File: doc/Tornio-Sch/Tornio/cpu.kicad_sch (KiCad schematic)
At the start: 24 parts, among them J3 Program, J5 Conn_02x20_Odd_Even, J7 Conn_02x07_Odd_Even, U10 STM32F103C6Tx, U2 ULN2003, U9 AMS1117-3.3, Y2 12MHz

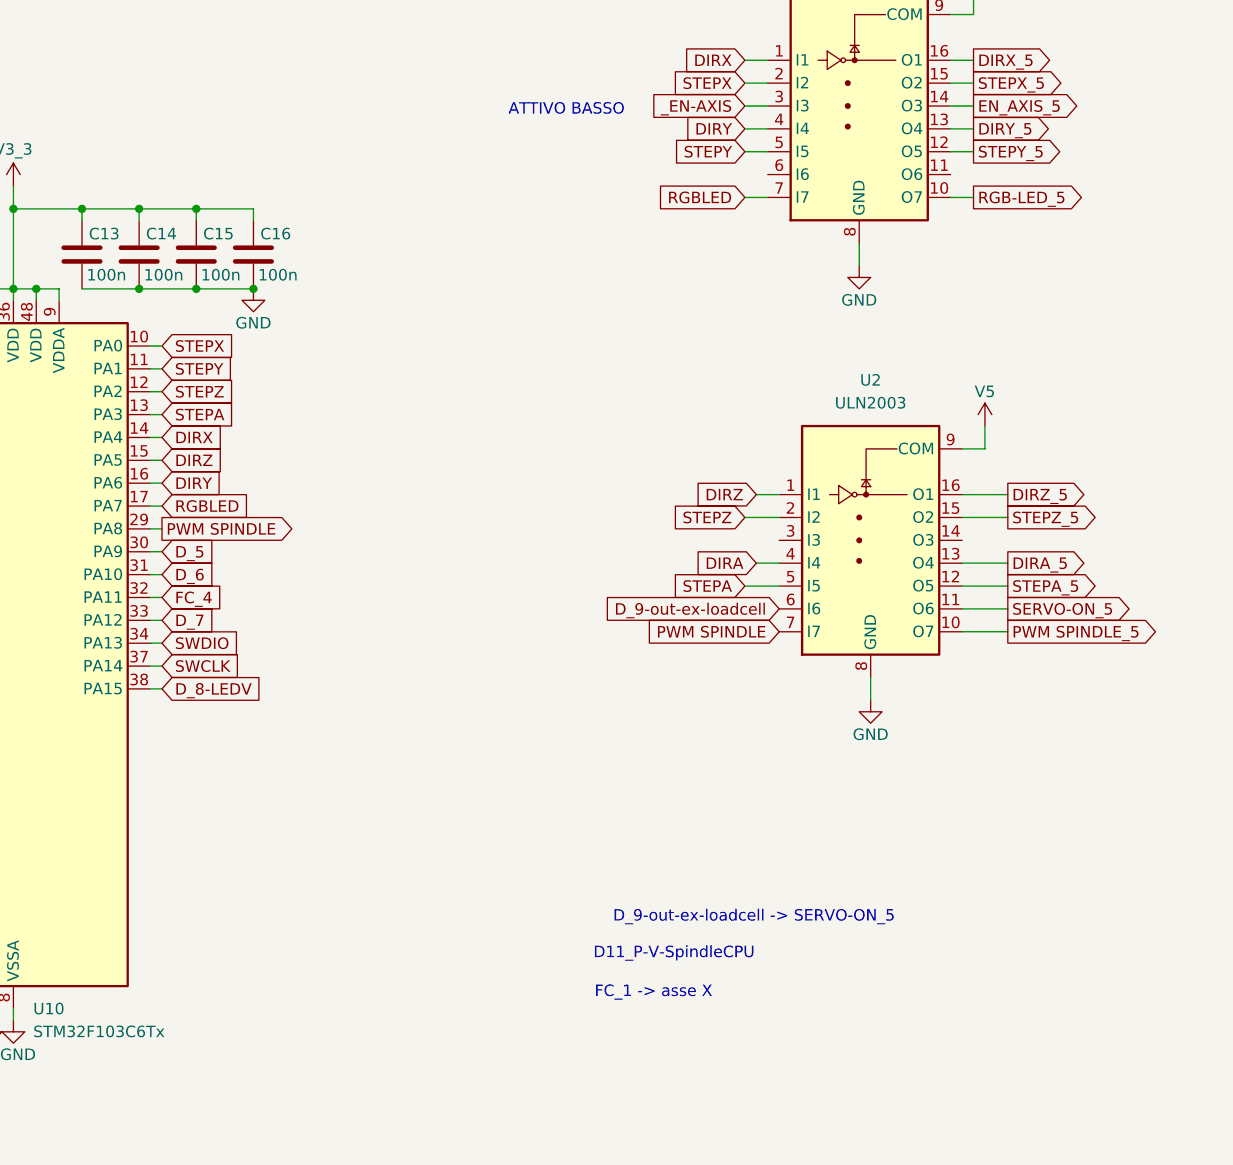
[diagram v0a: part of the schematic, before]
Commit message: eliminati file tenda da sole da accessori
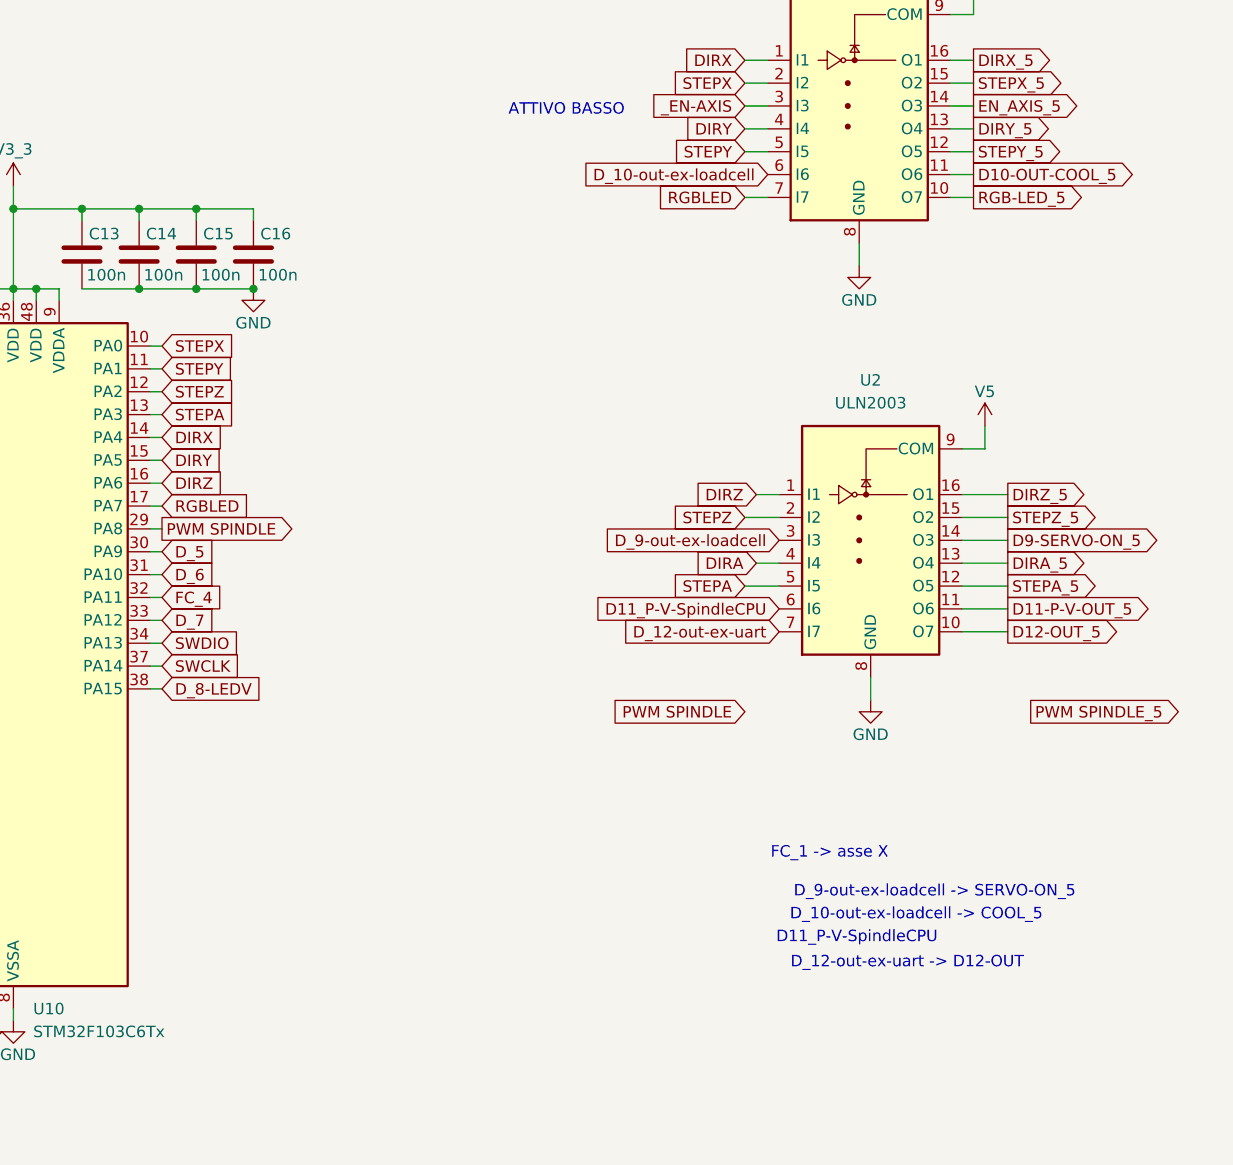
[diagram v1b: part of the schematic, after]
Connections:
- net D11_P-V-SpindleCPU: now also U2.6 (I6)
- net DIRY: now also U10.15 (PA5); no longer U10.16 (PA6)
- net DIRZ: now also U10.16 (PA6); no longer U10.15 (PA5)
- net D_10-out-ex-loadcell: now also U2.6 (I6)
- net D_12-out-ex-uart: now also U2.7 (I7)
- net D_9-out-ex-loadcell: now also U2.3 (I3); no longer U2.6 (I6)
- net PWM SPINDLE: no longer U2.7 (I7)
- net PWM SPINDLE_5: no longer U2.10 (O7)
- net D9-SERVO-ON_5: now reaches U2.14 (O3)
- net D10-OUT-COOL_5: now reaches U2.11 (O6)
- net SERVO-ON_5 renamed D11-P-V-OUT_5
- new net D12-OUT_5: U2.10 (O7)
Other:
- note added: "D_10-out-ex-loadcell -> COOL_5"
- note added: "D_12-out-ex-uart -> D12-OUT"
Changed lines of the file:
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@@
 	(generator_version "9.0")
 	(paper "A4")
+	(title_block
+		(date "2026-07-28")
+		(rev "1.0")
+	)
+	(text "D_9-out-ex-loadcell -> SERVO-ON_5"
+		(exclude_from_sim no)
+		(at 252.222 121.666 0)
+		(effects
+			(font
+				(size 1.27 1.27)
+			)
+		)
+	)
 	(text "GND pin 35 - 47"
 		(exclude_from_sim no)
@@
 	(text "FC_1 -> asse X"
 		(exclude_from_sim no)
-		(at 220.98 132.842 0)
+		(at 240.538 117.348 0)
 		(effects
 			(font
@@
 		)
 	)
-	(text "D_9-out-ex-loadcell -> SERVO-ON_5"
+	(text "D_12-out-ex-uart -> D12-OUT"
 		(exclude_from_sim no)
-		(at 232.156 124.46 0)
+		(at 249.174 129.54 0)
+		(effects
+			(font
+				(size 1.27 1.27)
+			)
+		)
+	)
+	(text "D_10-out-ex-loadcell -> COOL_5"
+		(exclude_from_sim no)
+		(at 250.19 124.206 0)
 		(effects
 			(font
@@
 	(text "D11_P-V-SpindleCPU"
 		(exclude_from_sim no)
-		(at 223.266 128.524 0)
+		(at 243.586 126.746 0)
 		(effects
 			(font
@@
 	(wire
 		(pts
+			(xy 256.54 41.91) (xy 254 41.91)
+		)
+		(stroke
+			(width 0)
+			(type default)
+		)
+	)
+	(wire
+		(pts
 			(xy 149.86 54.61) (xy 152.4 54.61)
 		)
@@
 	(wire
 		(pts
+			(xy 260.35 82.55) (xy 255.27 82.55)
+		)
+		(stroke
+			(width 0)
+			(type default)
+		)
+	)
+	(wire
+		(pts
 			(xy 255.27 90.17) (xy 260.35 90.17)
 		)
@@
 		)
 	)
+	(global_label "D11-P-V-OUT_5"
+		(shape output)
+		(at 260.35 90.17 0)
+		(fields_autoplaced yes)
+		(effects
+			(font
+				(size 1.27 1.27)
+			)
+			(justify left)
+		)
+		(property "Intersheetrefs" "${INTERSHEET_REFS}"
+			(at 279.9057 90.17 0)
+			(effects
+				(font
+					(size 1.27 1.27)
+				)
+				(justify left)
+				(hide yes)
+			)
+		)
+	)
 	(global_label "SPI2_MISO"
 		(shape input)
@@
 		)
 	)
-	(global_label "PWM SPINDLE"
-		(shape input)
-		(at 234.95 92.71 180)
-		(fields_autoplaced yes)
-		(effects
-			(font
-				(size 1.27 1.27)
-			)
-			(justify right)
-		)
-		(property "Intersheetrefs" "${INTERSHEET_REFS}"
-			(at 218.9625 92.71 0)
-			(effects
-				(font
-					(size 1.27 1.27)
-				)
-				(justify right)
-				(hide yes)
-			)
-		)
-	)
 	(global_label "SPI2_MOSI"
 		(shape input)
@@
 		)
 	)
-	(global_label "DIRY"
+	(global_label "DIRZ"
 		(shape input)
 		(at 166.37 76.2 0)
@@
 		)
 		(property "Intersheetrefs" "${INTERSHEET_REFS}"
-			(at 173.5886 76.2 0)
+			(at 173.7095 76.2 0)
 			(effects
 				(font
@@
 		)
 	)
-	(global_label "PWM SPINDLE_5"
-		(shape output)
-		(at 260.35 92.71 0)
+	(global_label "D_12-out-ex-uart"
+		(shape input)
+		(at 234.95 92.71 180)
 		(fields_autoplaced yes)
 		(effects
@@
 				(size 1.27 1.27)
 			)
-			(justify left)
+			(justify right)
 		)
 		(property "Intersheetrefs" "${INTERSHEET_REFS}"
-			(at 278.5146 92.71 0)
+			(at 213.6407 92.71 0)
 			(effects
 				(font
 					(size 1.27 1.27)
 				)
-				(justify left)
+				(justify right)
+				(hide yes)
+			)
+		)
+	)
+	(global_label "D11_P-V-SpindleCPU"
+		(shape input)
+		(at 234.95 90.17 180)
+		(fields_autoplaced yes)
+		(effects
+			(font
+				(size 1.27 1.27)
+			)
+			(justify right)
+		)
+		(property "Intersheetrefs" "${INTERSHEET_REFS}"
+			(at 210.9192 90.17 0)
+			(effects
+				(font
+					(size 1.27 1.27)
+				)
+				(justify right)
 				(hide yes)
 			)
@@
 		)
 	)
+	(global_label "D10-OUT-COOL_5"
+		(shape output)
+		(at 256.54 41.91 0)
+		(fields_autoplaced yes)
+		(effects
+			(font
+				(size 1.27 1.27)
+			)
+			(justify left)
+		)
+		(property "Intersheetrefs" "${INTERSHEET_REFS}"
+			(at 277.1238 41.91 0)
+			(effects
+				(font
+					(size 1.27 1.27)
+				)
+				(justify left)
+				(hide yes)
+			)
+		)
+	)
 	(global_label "SPI2_CLK"
 		(shape input)
@@
 		)
 	)
+	(global_label "D_10-out-ex-loadcell"
+		(shape input)
+		(at 233.68 41.91 180)
+		(fields_autoplaced yes)
+		(effects
+			(font
+				(size 1.27 1.27)
+			)
+			(justify right)
+		)
+		(property "Intersheetrefs" "${INTERSHEET_REFS}"
+			(at 208.5608 41.91 0)
+			(effects
+				(font
+					(size 1.27 1.27)
+				)
+				(justify right)
+				(hide yes)
+			)
+		)
+	)
 	(global_label "PWM SPINDLE"
 		(shape output)
@@
 		)
 	)
-	(global_label "FC_1"
+	(global_label "D_9-out-ex-loadcell"
 		(shape input)
-		(at 129.54 93.98 180)
+		(at 234.95 82.55 180)
 		(fields_autoplaced yes)
 		(effects
@@
 		)
 		(property "Intersheetrefs" "${INTERSHEET_REFS}"
-			(at 122.0191 93.98 0)
+			(at 211.0403 82.55 0)
 			(effects
 				(font
@@
 		)
 	)
-	(global_label "ADC2"
+	(global_label "FC_1"
 		(shape input)
-		(at 129.54 91.44 180)
+		(at 129.54 93.98 180)
 		(fields_autoplaced yes)
 		(effects
@@
 		)
 		(property "Intersheetrefs" "${INTERSHEET_REFS}"
-			(at 121.7167 91.44 0)
+			(at 122.0191 93.98 0)
 			(effects
 				(font
@@
 		)
 	)
-	(global_label "D_9-out-ex-loadcell"
+	(global_label "ADC2"
 		(shape input)
-		(at 234.95 90.17 180)
+		(at 129.54 91.44 180)
 		(fields_autoplaced yes)
 		(effects
@@
 		)
 		(property "Intersheetrefs" "${INTERSHEET_REFS}"
-			(at 211.0403 90.17 0)
+			(at 121.7167 91.44 0)
 			(effects
 				(font
@@
 		)
 	)
+	(global_label "D12-OUT_5"
+		(shape output)
+		(at 260.35 92.71 0)
+		(fields_autoplaced yes)
+		(effects
+			(font
+				(size 1.27 1.27)
+			)
+			(justify left)
+		)
+		(property "Intersheetrefs" "${INTERSHEET_REFS}"
+			(at 274.4023 92.71 0)
+			(effects
+				(font
+					(size 1.27 1.27)
+				)
+				(justify left)
+				(hide yes)
+			)
+		)
+	)
 	(global_label "DIRA"
 		(shape input)
@@
 		)
 	)
+	(global_label "PWM SPINDLE_5"
+		(shape output)
+		(at 262.89 101.6 0)
+		(fields_autoplaced yes)
+		(effects
+			(font
+				(size 1.27 1.27)
+			)
+			(justify left)
+		)
+		(property "Intersheetrefs" "${INTERSHEET_REFS}"
+			(at 281.0546 101.6 0)
+			(effects
+				(font
+					(size 1.27 1.27)
+				)
+				(justify left)
+				(hide yes)
+			)
+		)
+	)
 	(global_label "ENC_CLK"
 		(shape input)
@@
 		)
 	)
-	(global_label "SERVO-ON_5"
+	(global_label "D9-SERVO-ON_5"
 		(shape output)
-		(at 260.35 90.17 0)
+		(at 260.35 82.55 0)
 		(fields_autoplaced yes)
 		(effects
@@
 		)
 		(property "Intersheetrefs" "${INTERSHEET_REFS}"
-			(at 275.7933 90.17 0)
+			(at 279.8452 82.55 0)
 			(effects
 				(font
@@
 		)
 	)
+	(global_label "PWM SPINDLE"
+		(shape input)
+		(at 231.14 101.6 180)
+		(fields_autoplaced yes)
+		(effects
+			(font
+				(size 1.27 1.27)
+			)
+			(justify right)
+		)
+		(property "Intersheetrefs" "${INTERSHEET_REFS}"
+			(at 215.1525 101.6 0)
+			(effects
+				(font
+					(size 1.27 1.27)
+				)
+				(justify right)
+				(hide yes)
+			)
+		)
+	)
 	(global_label "FC_2"
 		(shape input)
@@
 		)
 	)
-	(global_label "DIRZ"
+	(global_label "DIRY"
 		(shape input)
 		(at 166.37 73.66 0)
@@
 		)
 		(property "Intersheetrefs" "${INTERSHEET_REFS}"
-			(at 173.7095 73.66 0)
+			(at 173.5886 73.66 0)
 			(effects
 				(font
